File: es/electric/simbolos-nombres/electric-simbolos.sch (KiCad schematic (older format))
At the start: 87 parts, among them J1 conector, K1 CONTACTO, K1 RELE, M1 MOTOR, Q1 TRANSISTOR, Q2 TRANSISTOR, U1 AO, U1 logic_and, U2 logic_and, U3 logic_and, U4 logic_and, U5 logic_and, U6 logic_and

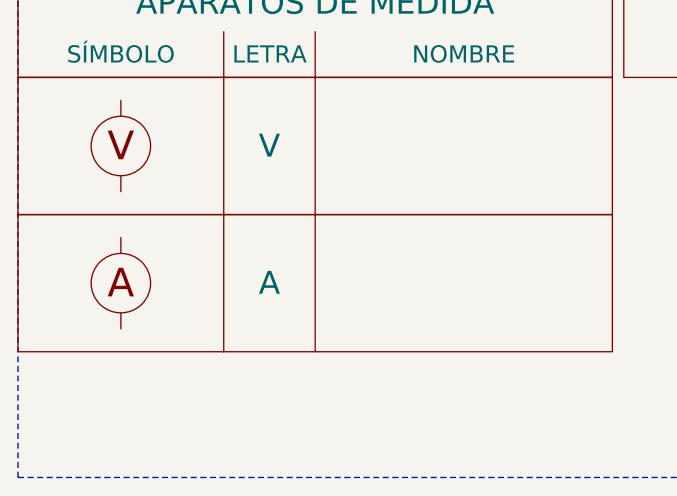
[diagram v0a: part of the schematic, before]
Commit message: Cambios a 23/05/2022.
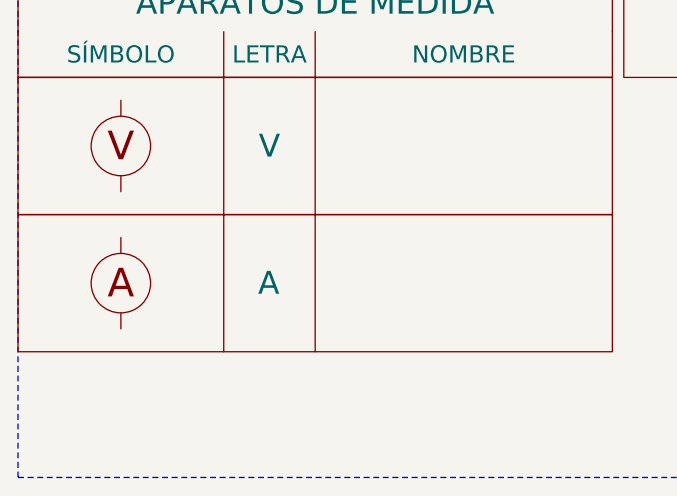
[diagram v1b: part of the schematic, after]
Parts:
- removed A: AMPERIMETRO, symbol electric-simbolos-nombres-rescue:amperimetro-simbolos
- added A: amperimetro, symbol simbolos:amperimetro
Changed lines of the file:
@@
-$EndComp
-$Comp
-L electric-simbolos-nombres-rescue:amperimetro-simbolos A
-U 1 1 5BC41F8F
-P 650 10450
-AR Path="/5BC41F8F" Ref="A"  Part="1"
-AR Path="/5BC9CE01/5BC41F8F" Ref="A"  Part="1"
-F 0 "A" H 1300 10250 100 0000 C CNN
-F 1 "AMPERIMETRO" H 1600 10250 100 0001 L CNN
-F 2 "" V 650 10225 50  0001 C CNN
-F 3 "" V 650 10225 50  0001 C CNN
-	1    650  10450
-	1    0    0    -1
 $EndComp
 $Comp
@@
 	1    0    0    -1
 $EndComp
+$Comp
+L simbolos:amperimetro A?
+U 1 1 628C28C8
+P 650 10450
+AR Path="/628C28C8" Ref="A?"  Part="1"
+AR Path="/5BC9CE01/628C28C8" Ref="A"  Part="1"
+F 0 "A" H 1250 10250 100 0000 L CNN
+F 1 "amperimetro" V 500 10250 50  0001 C CNN
+F 2 "" V 650 10225 50  0001 C CNN
+F 3 "" V 650 10225 50  0001 C CNN
+	1    650  10450
+	1    0    0    -1
+$EndComp
